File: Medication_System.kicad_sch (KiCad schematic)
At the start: 25 parts, among them J1 USB_C_Receptacle_USB2.0_14P, M1 Motor_Servo, M2 Motor_Servo, M3 Motor_Servo, M4 Motor_Servo, U1 AMS1117-3.3, U2 ESP32-C6-MINI-1, U3 RC1602A-GHW-ESX

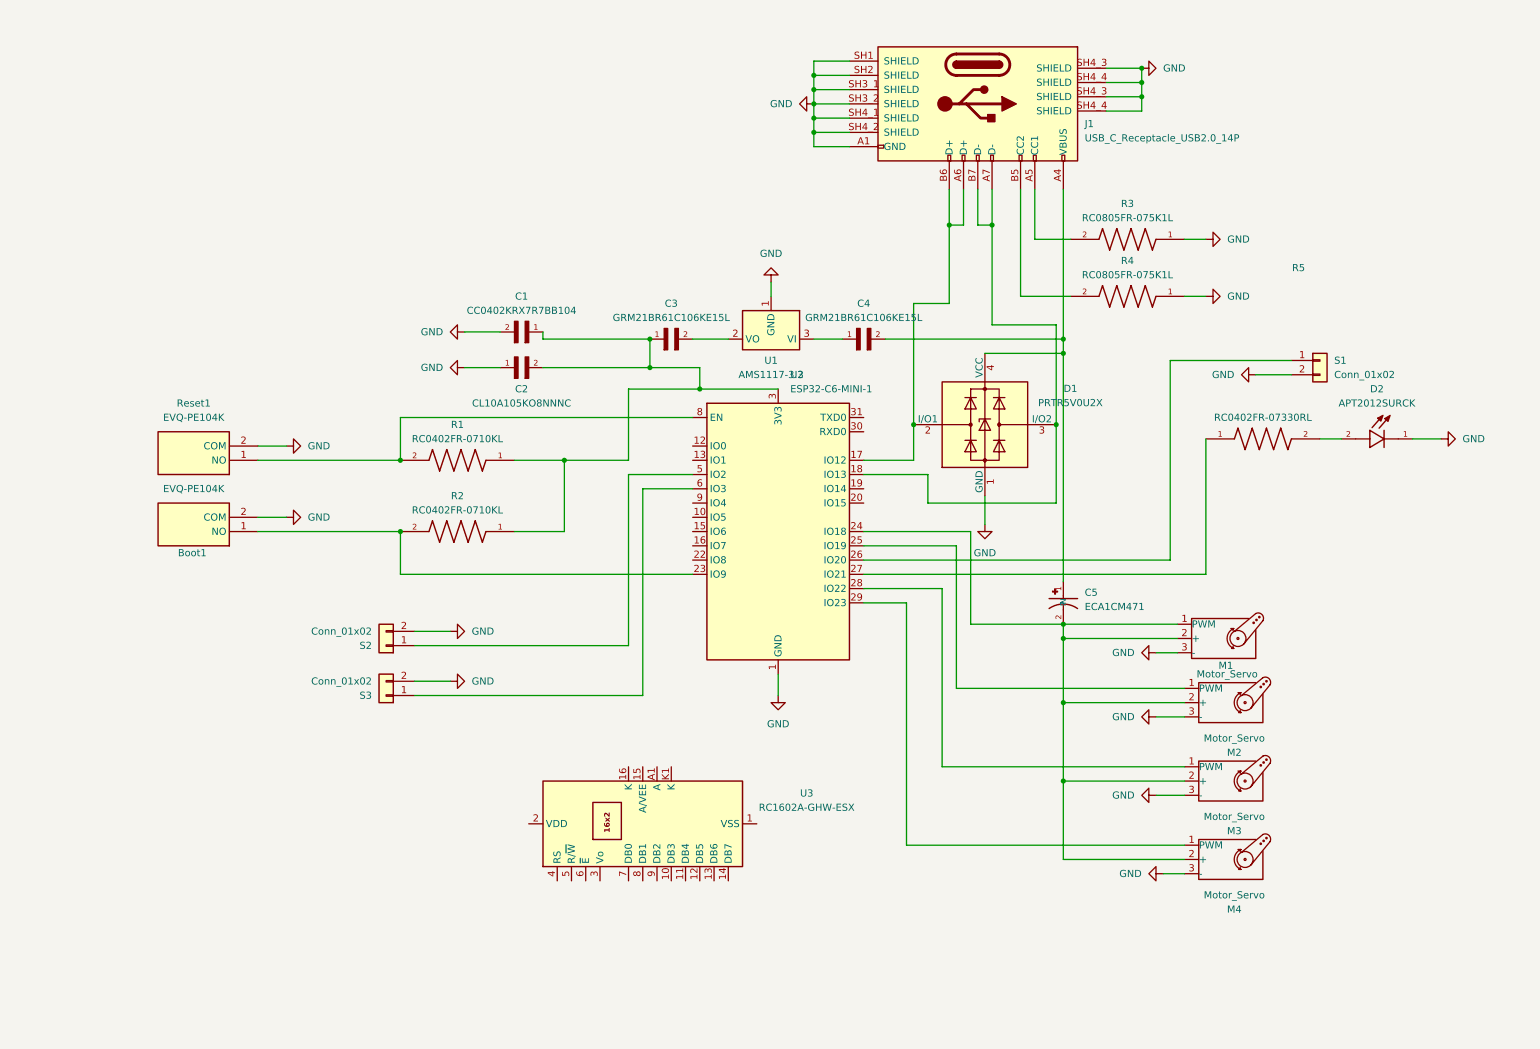
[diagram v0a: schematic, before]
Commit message: Snapshot of pre-final S3/stepper work before reorganizing
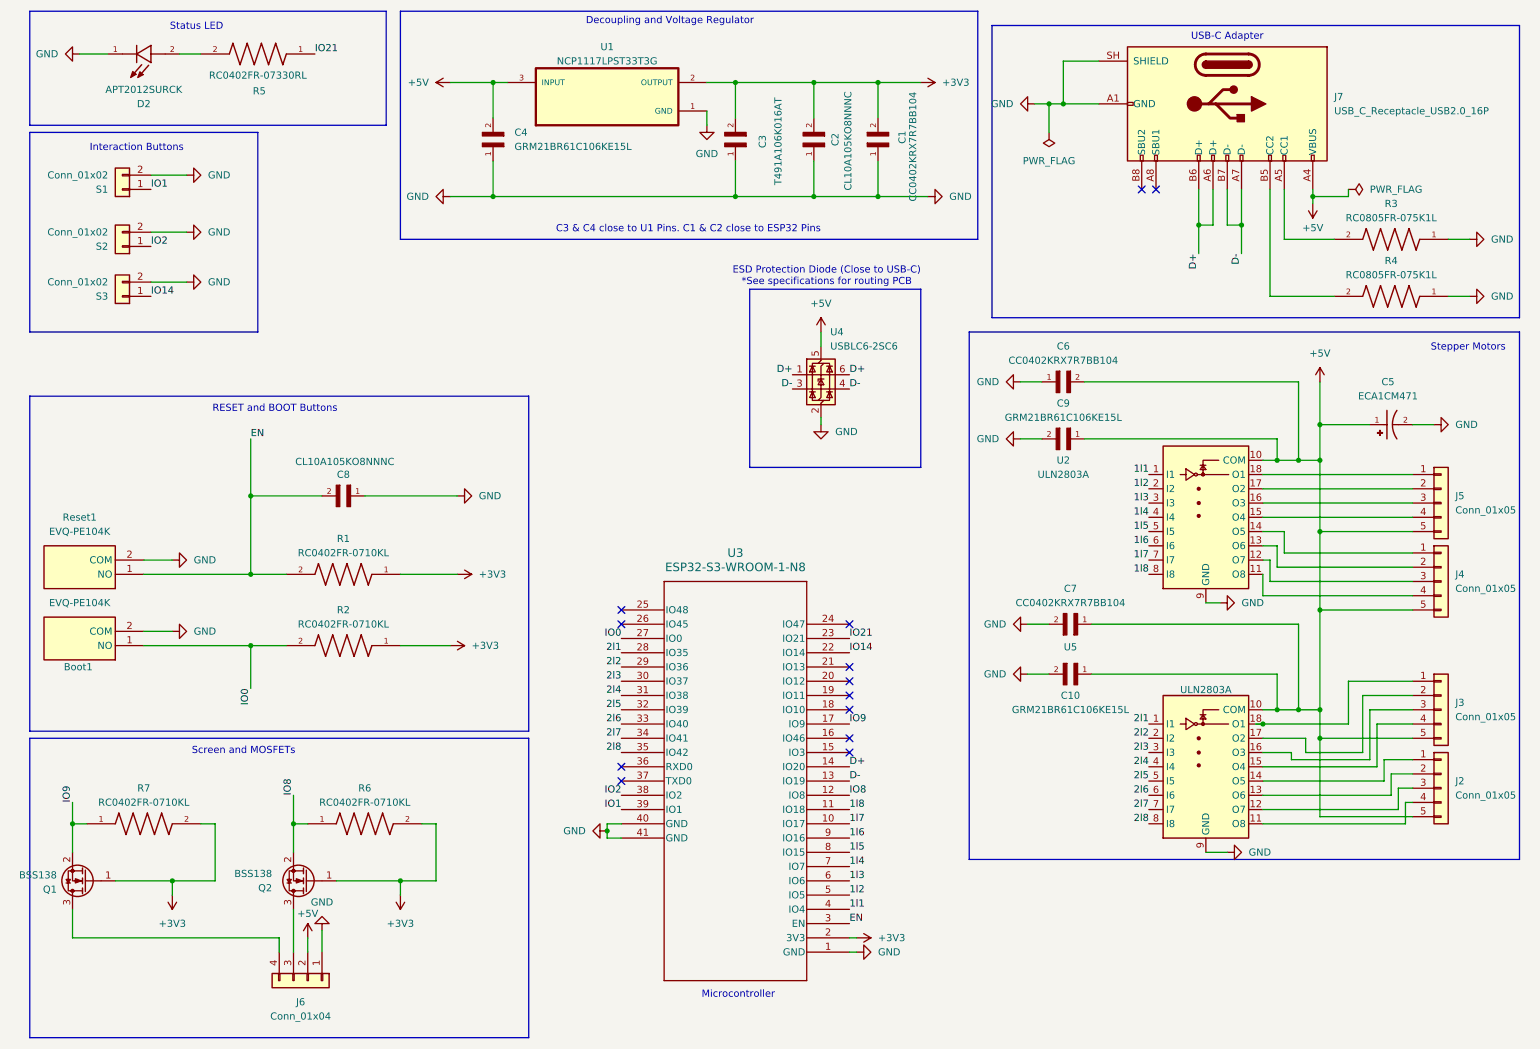
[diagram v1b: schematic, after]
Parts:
- removed C3: GRM21BR61C106KE15L, GRM21BR61C106KE15L:CAPC2012X135N, symbol GRM21BR61C106KE15L:GRM21BR61C106KE15L
- removed D1: PRTR5V0U2X, Package_TO_SOT_SMD:SOT-143, symbol Power_Protection:PRTR5V0U2X
- removed J1: USB_C_Receptacle_USB2.0_14P, 12401899E412A:AMPHENOL_12401899E412A, symbol Connector:USB_C_Receptacle_USB2.0_14P
- removed M1, M2, M3, M4: Motor_Servo, Connector_PinHeader_2.54mm:PinHeader_1x03_P2.54mm_Vertical, symbol Motor:Motor_Servo
- removed U1: AMS1117-3.3, Package_TO_SOT_SMD:SOT-223-3_TabPin2, symbol Regulator_Linear:AMS1117-3.3
- removed U2: ESP32-C6-MINI-1, RF_Module:ESP32-C6-MINI-1, symbol RF_Module:ESP32-C6-MINI-1
- removed U3: RC1602A-GHW-ESX, Display:RC1602A, symbol Display_Character:RC1602A-GHW-ESX
- added C10, C9: GRM21BR61C106KE15L, GRM21BR61C106KE15L:CAPC2012X135N, symbol GRM21BR61C106KE15L:GRM21BR61C106KE15L
- added C3: T491A106K016AT, T491A106K016AT:RESC3216X125N, symbol T491A106K016AT:T491A106K016AT
- added C6, C7: CC0402KRX7R7BB104, CC0402KRX7R7BB104:CAPC1005X55N, symbol CC0402KRX7R7BB104:CC0402KRX7R7BB104
- added C8: CL10A105KO8NNNC, CL10A105KO8NNNC:CAPC1608X90N, symbol CL10A105KO8NNNC:CL10A105KO8NNNC
- added J2, J3, J4, J5: Conn_01x05, Connector_JST:JST_XH_B5B-XH-A_1x05_P2.50mm_Vertical, symbol Connector_Generic:Conn_01x05
- added J6: Conn_01x04, Connector_JST:JST_XH_B4B-XH-A_1x04_P2.50mm_Vertical, symbol Connector_Generic:Conn_01x04
- added J7: USB_C_Receptacle_USB2.0_16P, Connector_USB:USB_C_Receptacle_GCT_USB4105-xx-A_16P_TopMnt_Horizontal, symbol Connector:USB_C_Receptacle_USB2.0_16P
- added Q1, Q2: BSS138, Package_TO_SOT_SMD:SOT-23, symbol Transistor_FET:BSS138
- added R6, R7: RC0402FR-0710KL, RC0402FR-0710KL:RESC1005X40N, symbol RC0402FR-0710KL:RC0402FR-0710KL
- added U1: NCP1117LPST33T3G, NCP1117LPST33T3G:SOT230P700X175-4N, symbol NCP1117LPST33T3G:NCP1117LPST33T3G
- added U2, U5: ULN2803A, Package_SO:SOIC-18W_7.5x11.6mm_P1.27mm, symbol Transistor_Array:ULN2803A
- added U3: ESP32-S3-WROOM-1-N8, RF_Module:ESP32-S3-WROOM-1, symbol ESP32-S3-WROOM-1-N8:ESP32-S3-WROOM-1-N8
- added U4: USBLC6-2SC6, Package_TO_SOT_SMD:SOT-23-6, symbol Power_Protection:USBLC6-2SC6
- R3, R4: footprint Resistor_SMD:R_0805_2012Metric -> Resistor_SMD:R_0805_2012Metric_Pad1.20x1.40mm_HandSolder
- S1, S2, S3: footprint Connector:JWT_A3963_1x02_P3.96mm_Vertical -> Connector_JST:JST_XH_B2B-XH-A_1x02_P2.50mm_Vertical
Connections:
- net GND: now also C1.1, C4.1, C5.2, C10.2, C3.1, C6.1, C7.2, C8.1, C9.2, J6.1 (Pin_1), J7.A1 (GND), J7.A12 (GND), J7.B1 (GND), J7.B12 (GND), J7.SH (SHIELD), U1.1 (GND), U2.9 (GND), U3.1 (GND), U3.40 (GND), U3.41 (GND), U4.2 (GND), U5.9 (GND); no longer C1.2
- net IO2: now reaches S2.1 (Pin_1)
- net IO2: now also U3.38 (IO2)
- net +3V3: now reaches C2.2, R1.1, R2.1
- net +3V3: now also C1.2, C3.2, Q1.1 (G), Q2.1 (G), R6.2, R7.2, U1.2 (OUTPUT), U1.4 (OUTPUT), U3.2 (3V3); no longer C1.1
- net IO0: now reaches Boot1.1 (NO), R2.2
- net IO0: now also U3.27 (IO0)
- net IO1: now reaches S1.1 (Pin_1)
- net IO1: now also U3.39 (IO1)
- net IO21: now reaches R5.1
- net IO21: now also U3.23 (IO21)
- net IO14: now reaches S3.1 (Pin_1)
- net IO14: now also U3.22 (IO14)
- net EN: now reaches R1.2, Reset1.1 (NO)
- net EN: now also C8.2, U3.3 (EN)
- net at R4.2: now also J7.B5 (CC2)
- net +5V: now reaches C4.2, C5.1
- net +5V: now also C10.1, C6.2, C7.1, C9.1, J2.5 (Pin_5), J3.5 (Pin_5), J4.5 (Pin_5), J5.5 (Pin_5), J6.2 (Pin_2), J7.A4 (VBUS), J7.A9 (VBUS), J7.B4 (VBUS), J7.B9 (VBUS), U1.3 (INPUT), U2.10 (COM), U4.5 (VBUS), U5.10 (COM)
- net at R3.2: now also J7.A5 (CC1)
- new net: J4.4 (Pin_4), U2.11 (O8)
- new net: J4.3 (Pin_3), U2.12 (O7)
- new net: J4.2 (Pin_2), U2.13 (O6)
- new net: J4.1 (Pin_1), U2.14 (O5)
- new net: J5.4 (Pin_4), U2.15 (O4)
- new net: J5.3 (Pin_3), U2.16 (O3)
- new net: J5.2 (Pin_2), U2.17 (O2)
- new net: J5.1 (Pin_1), U2.18 (O1)
- new net: J2.4 (Pin_4), U5.11 (O8)
- new net: J2.3 (Pin_3), U5.12 (O7)
- new net: J2.2 (Pin_2), U5.13 (O6)
- new net: J2.1 (Pin_1), U5.14 (O5)
- new net: J3.4 (Pin_4), U5.15 (O4)
- new net: J3.3 (Pin_3), U5.16 (O3)
- new net: J3.2 (Pin_2), U5.17 (O2)
- new net: J3.1 (Pin_1), U5.18 (O1)
- new net: J6.3 (Pin_3), Q2.3 (D)
- new net: J6.4 (Pin_4), Q1.3 (D)
- new net 1l1: U2.1 (I1), U3.4 (IO4)
- new net 1l2: U2.2 (I2), U3.5 (IO5)
- new net 1l3: U2.3 (I3), U3.6 (IO6)
- new net 1l4: U2.4 (I4), U3.7 (IO7)
- new net 1l5: U2.5 (I5), U3.8 (IO15)
- new net 1l6: U2.6 (I6), U3.9 (IO16)
- new net 1l7: U2.7 (I7), U3.10 (IO17)
- new net 1l8: U2.8 (I8), U3.11 (IO18)
- new net 2l1: U3.28 (IO35), U5.1 (I1)
- new net 2l2: U3.29 (IO36), U5.2 (I2)
- new net 2l3: U3.30 (IO37), U5.3 (I3)
- new net 2l4: U3.31 (IO38), U5.4 (I4)
- new net 2l5: U3.32 (IO39), U5.5 (I5)
- new net 2l6: U3.33 (IO40), U5.6 (I6)
- new net 2l7: U3.34 (IO41), U5.7 (I7)
- new net 2l8: U3.35 (IO42), U5.8 (I8)
- new net D+: J7.A6 (D+), J7.B6 (D+), U3.14 (IO20), U4.1 (I/O1), U4.6 (I/O1)
- new net D-: J7.A7 (D-), J7.B7 (D-), U3.13 (IO19), U4.3 (I/O2), U4.4 (I/O2)
- new net IO8: Q2.2 (S), R6.1, U3.12 (IO8)
- new net IO9: Q1.2 (S), R7.1, U3.17 (IO9)
- no-connect marks 0 -> 13
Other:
- note added: "C3 & C4 close to U1 Pins. C1 & C2 close to ESP32 Pins"
- note added: "Decoupling and Voltage Regulator"
- note added: "ESD Protection Diode (Close to USB-C) *See specifications for routing PCB"
- note added: "Interaction Buttons"
- note added: "Microcontroller"
- note added: "RESET and BOOT Buttons"
- note added: "Screen and MOSFETs"
- note added: "Status LED"
- note added: "Stepper Motors"
- note added: "USB-C Adapter"
- moved on the sheet: Boot1, D2, R1, R2, R3, R4, R5, Reset1, S1, S2, S3
